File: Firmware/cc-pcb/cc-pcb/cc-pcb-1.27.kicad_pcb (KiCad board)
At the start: 2 copper layers, 31.5 x 36.8 mm, 25 parts, among them CON1 BARREL_JACK, IC1 ATMEGA328P-A, P1 CONN_20, P10 CONN_1, P11 CONN_1, P2 CONN_2, P4 CONN_1, P5 CONN_1, P6 CONN_1, P7 CONN_1, P8 CONN_1, P9 CONN_1, SW1 SRS

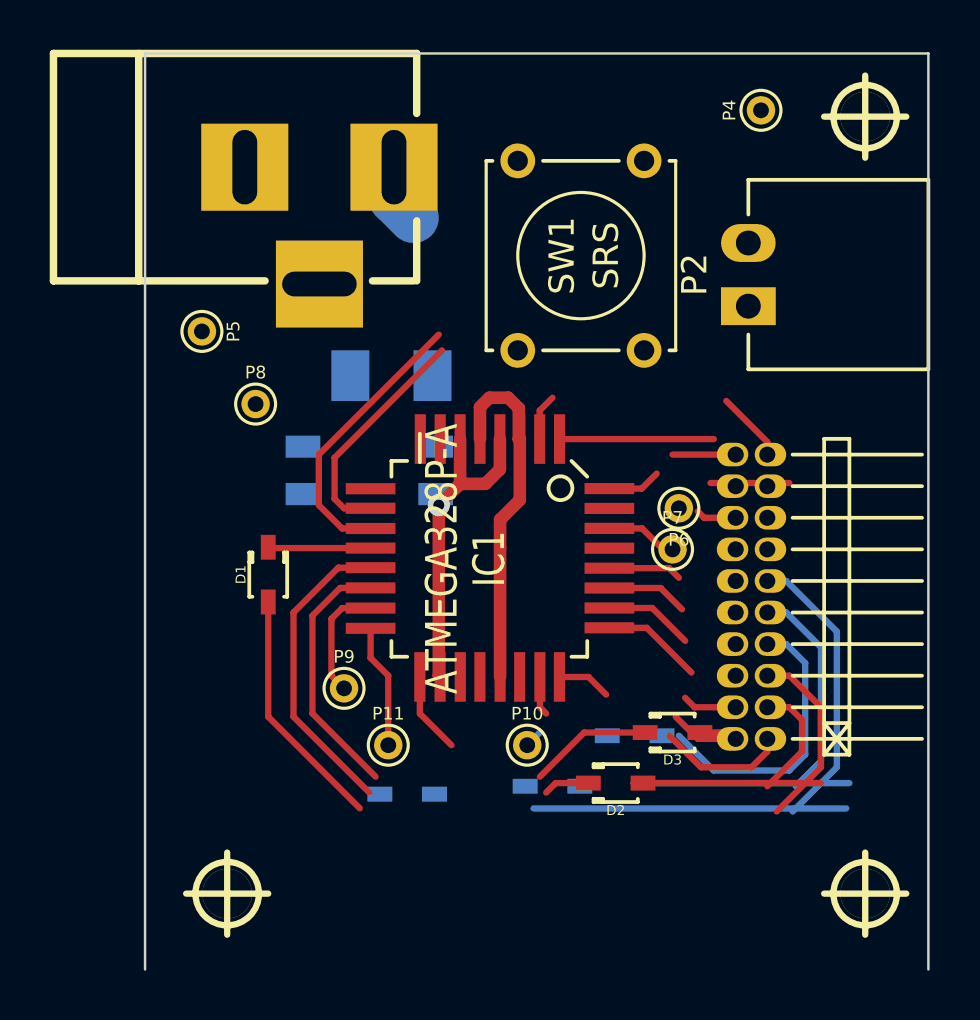
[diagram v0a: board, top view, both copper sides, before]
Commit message: in the middle of routing...
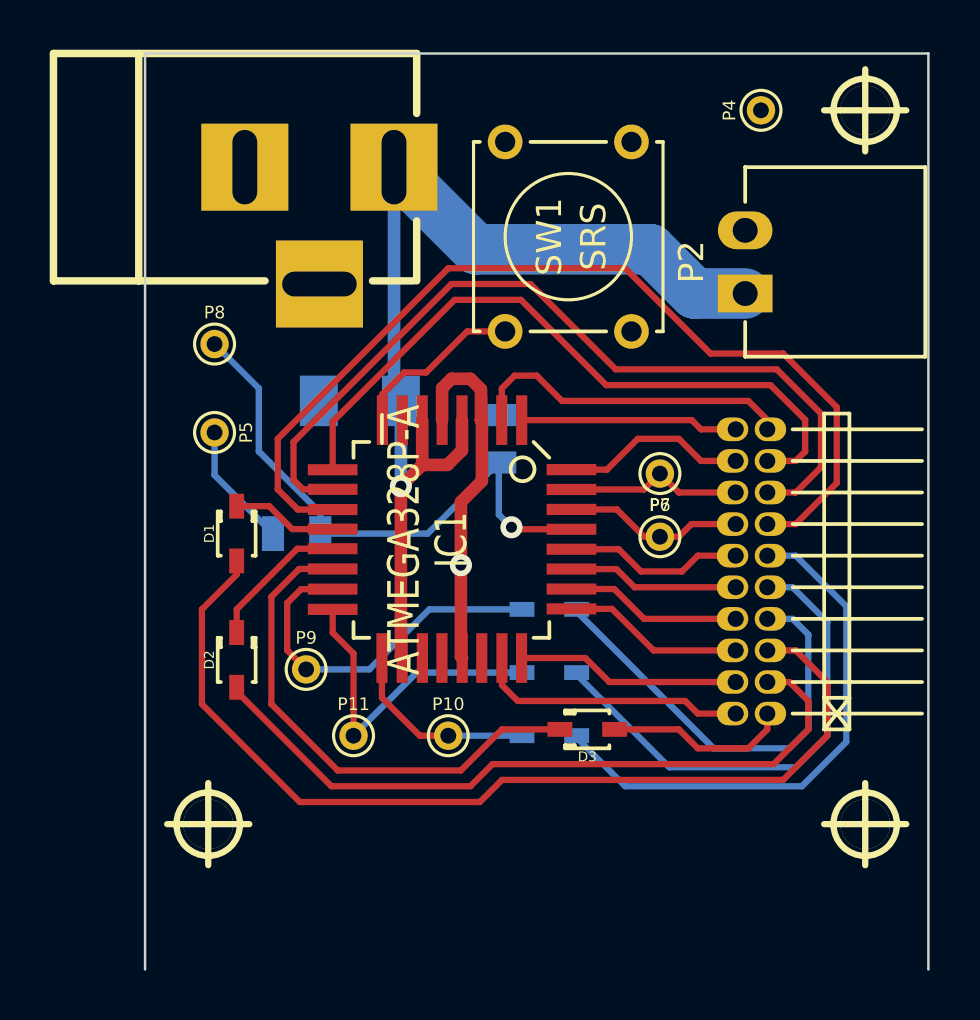
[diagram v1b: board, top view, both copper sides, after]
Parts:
- moved D2 16.0 mm to (103.8, 124.5), turned to 90 degrees
- moved D4 9.37 mm to (116.3, 122.4)
- moved D5 4.57 mm to (116.3, 125.0)
- moved P5 4.10 mm to (102.9, 115.3)
- moved D3 3.43 mm to (117.9, 127.3)
- moved D6 3.43 mm to (116.3, 127.5)
- moved P10 3.20 mm to (112.3, 127.5)
- moved P8 2.92 mm to (102.9, 111.8)
- moved H3 2.90 mm to (102.6, 131.1)
- moved R1 2.84 mm to (114.3, 115.6)
- moved H2 2.79 mm to (129.0, 131.1)
- moved C2 2.55 mm to (106.2, 119.4), turned to 180 degrees
- moved D1 2.08 mm to (103.8, 119.4)
- moved IC1 1.70 mm to (112.4, 119.6)
- moved P9 1.70 mm to (106.6, 124.8)
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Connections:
- D4 pad 1: N-0000019 (its old number) -> N-0000022
- D6 pad 1: N-0000020 (its old number) -> N-0000023
- P1 pad 11: N-0000019 (its old number) -> N-0000023
- P1 pad 7: N-0000020 (its old number) -> N-0000022
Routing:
- net N-0000030: track 0.00 -> 27.9 mm
- net N-0000033: track 11.3 -> 38.7 mm
- net VCC: track 15.4 -> 42.2 mm, vias 0 -> 1
- net N-0000031: track 9.36 -> 34.0 mm
- net (no net): track 24.4 -> 0.00 mm
- net N-0000011: track 0.00 -> 23.0 mm
- net N-0000023: track 0.00 -> 21.9 mm
- net N-0000015: track 17.4 -> 39.3 mm
- net N-0000022: track 0.00 -> 17.7 mm
- net N-0000014: track 12.0 -> 28.8 mm
- net N-0000019 (its old number): track 11.6 -> 0.00 mm
- net N-0000020 (its old number): track 11.4 -> 0.00 mm
- net N-0000018: track 8.75 -> 19.8 mm
- net N-000008: track 4.76 -> 14.7 mm
- net N-0000021: track 2.26 -> 11.0 mm
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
